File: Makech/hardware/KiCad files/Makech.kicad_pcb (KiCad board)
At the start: 2 copper layers, 55 x 110.1 mm, 99 parts, among them IC1 ULN2803, J1 SWD programmer, J2 USB_B_Micro, J3 ESP32-Exp, SW1 RST, SW2 SW_DPDT_x2, U1 ATSAMD21G18A-AU, U2 CONN_01X04, U3 AP2114_3.3v, X1 Screw_Terminal_1x02

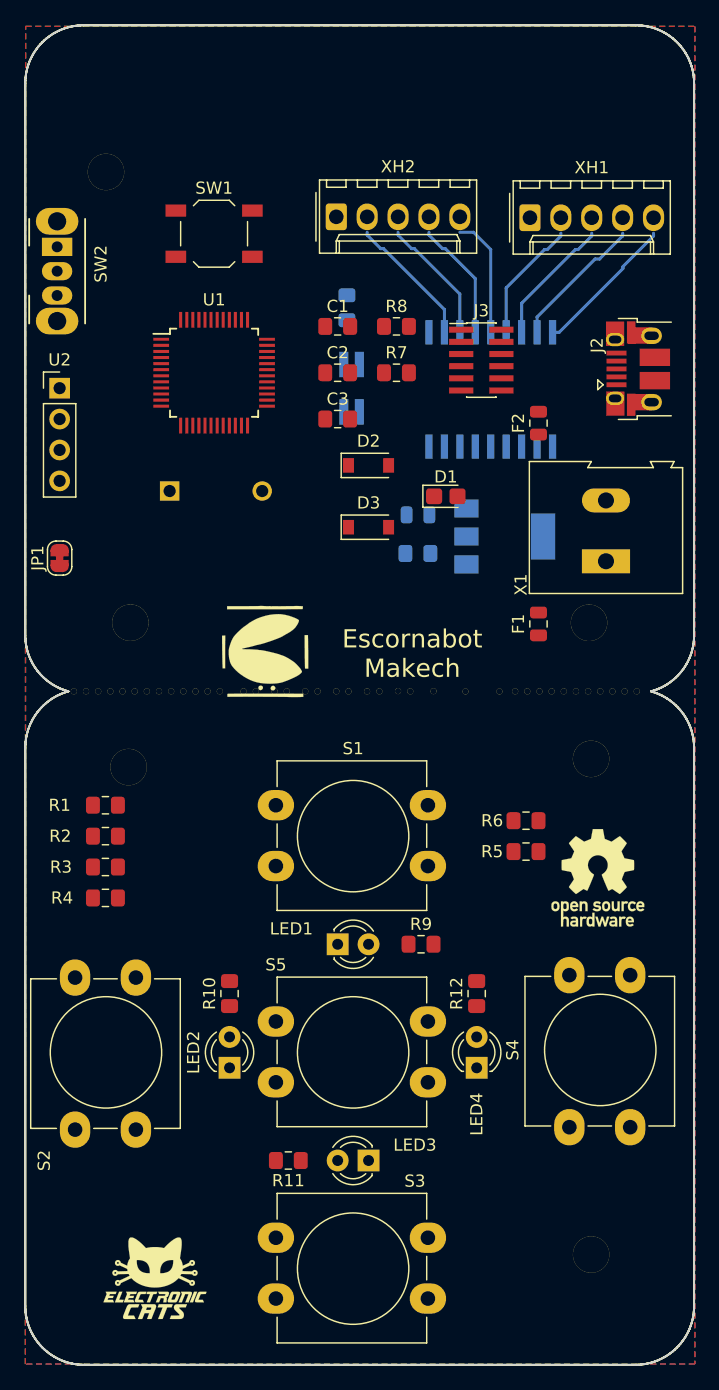
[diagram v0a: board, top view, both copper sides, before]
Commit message: fix pcb
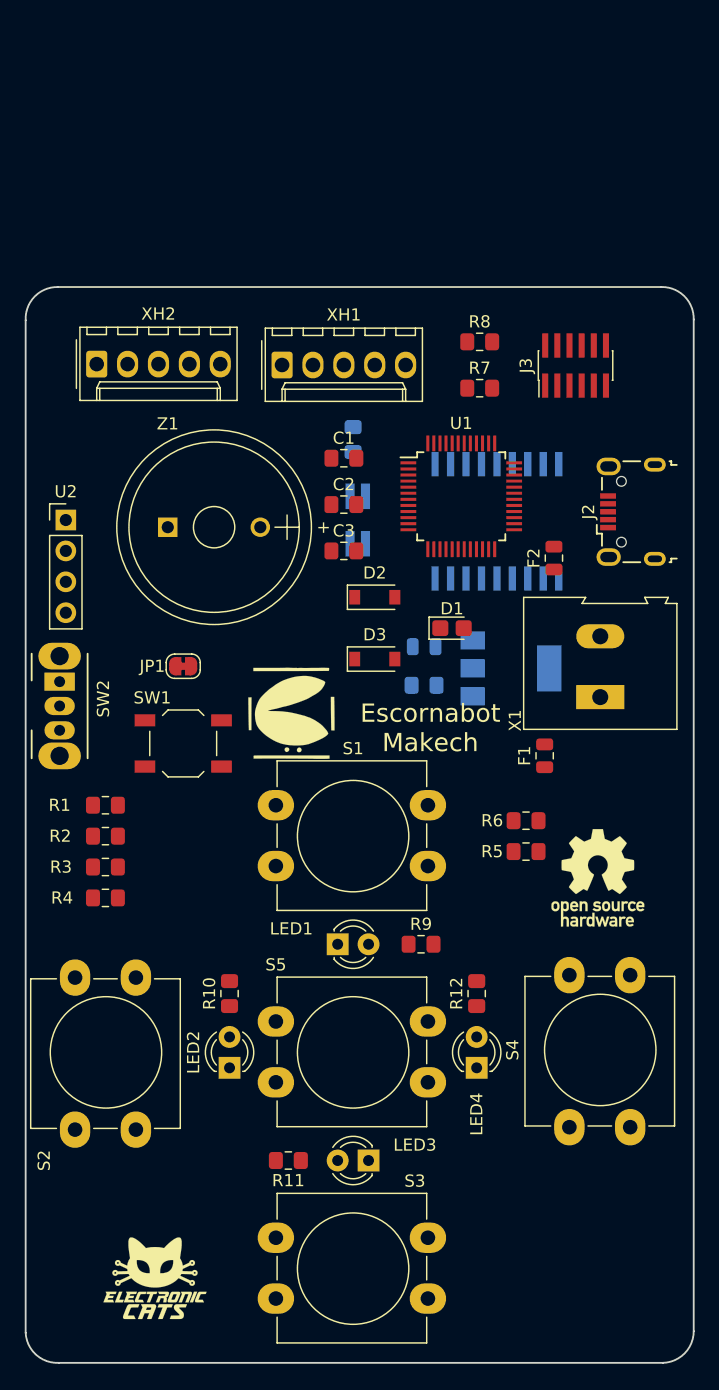
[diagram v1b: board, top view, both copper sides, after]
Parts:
- removed ? (x6): hole, ComponentesVarios:hole_3mm
- removed ? (x39): , ComponentesVarios:hole_05mm
- removed svg2mod: G***, borde:svg2mod
- removed svg2mod: G***, borde_S:svg2mod
- J2: footprint Connector_USB:USB_Micro-B_Amphenol_10103594-0001LF_Horizontal -> Connector_USB:USB_Micro-B_Wuerth_629105150521
- Z1: moved to F.Cu
- moved SW1 42.0 mm to (110.5, 94.0)
- moved SW2 35.8 mm to (100.3, 88.9)
- moved XH1 23.7 mm to (118.6, 62.9)
- moved XH2 23.1 mm to (103.4, 62.8)
- moved U1 22.7 mm to (133.3, 73.7)
- moved JP1 13.5 mm to (110.5, 87.6), turned to 180 degrees
- moved J2 11.8 mm to (147.3, 74.9)
- moved X1 11.2 mm to (144.8, 90.2)
- moved F2 11.2 mm to (141.0, 78.7)
- moved C1 10.9 mm to (123.7, 70.5)
- moved C2 10.9 mm to (123.7, 74.3)
- moved C3 10.9 mm to (123.7, 78.2)
- moved C4 10.9 mm to (130.3, 89.2)
- moved C6 10.9 mm to (124.5, 69.0)
- moved D3 10.9 mm to (126.2, 87.0)
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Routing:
- net /ML1: track 11.9 -> 0.00 mm
- net /ML2: track 11.3 -> 0.00 mm
- net /MR4: track 11.0 -> 0.00 mm
- net /ML3: track 10.7 -> 0.00 mm
- net /MR3: track 10.5 -> 0.00 mm
- net /ML4: track 10.1 -> 0.00 mm
- net /MR2: track 9.94 -> 0.00 mm
- net /MR1: track 9.93 -> 0.00 mm
- removed copper zone on B.Cu, net GND
- removed copper zone on F.Cu, net GND
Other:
- board size 55 x 110.1 mm -> 54.9 x 88.5 mm
